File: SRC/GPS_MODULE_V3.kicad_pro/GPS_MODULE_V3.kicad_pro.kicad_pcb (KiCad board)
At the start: 4 copper layers, 50.1 x 41 mm, 141 parts, among them J1 Input, J3 nano_sim, J4 Micro_SD_Card, J5 Conn_02x06_Counter_Clockwise, Q1 SSM3J328R-HXY, Q2 BSN20, Q3 BSN20, Q4 2N7002, Q5 2N7002, Q6 2N7002, Q7 2N7002, U1 SY8089AAAC, U2 STM32F103C8Tx, U3 A9G_MODULE, U4 MAX485E, U5 XC6206PxxxMR, U7 ATA6561-GAQW-N, U8 W25Q32JVSS, Y1 8MHz, Y2 32.678KHz

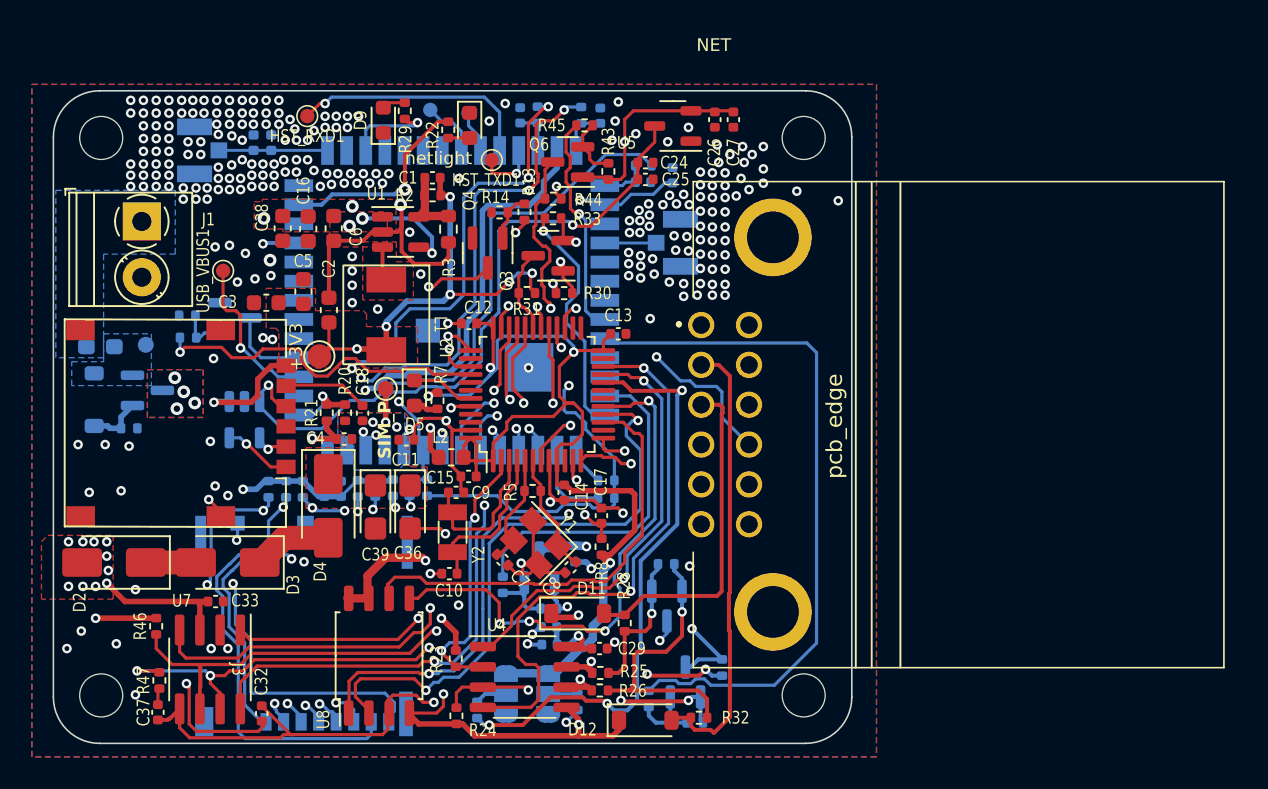
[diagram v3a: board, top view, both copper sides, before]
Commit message: completed GPS ecoboda files
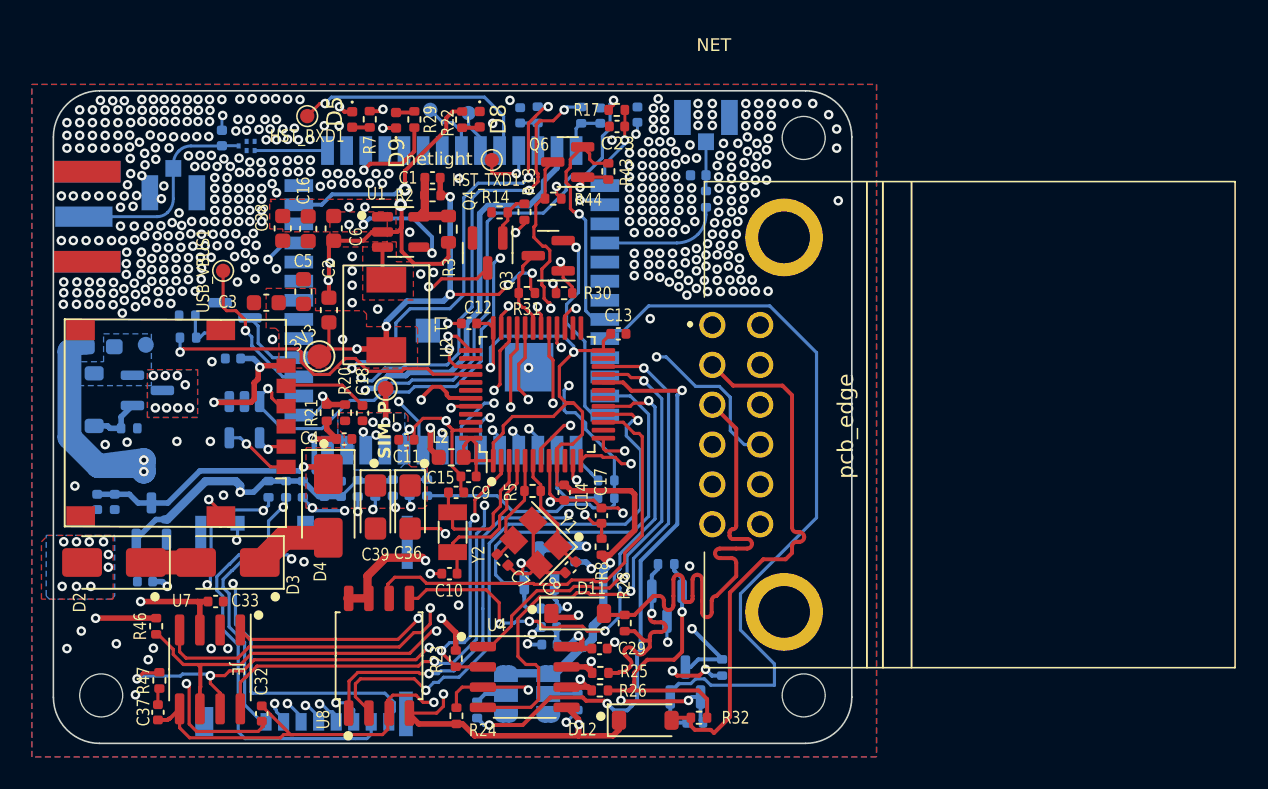
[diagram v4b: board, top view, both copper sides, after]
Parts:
- removed H2: MountingHole, MountingHole:MountingHole_2.7mm
- removed J1: Input, TerminalBlock_Phoenix:TerminalBlock_Phoenix_PT-1,5-2-3.5-H_1x02_P3.50mm_Horizontal
- removed R33, R36, R45, R50: 1K, Resistor_SMD:R_0402_1005Metric
- added AE3: Antenna_Shield, greencharge-footprints:UFL_COAX_CONN23370191, B.Cu at (230.9, 72.4)
- added C19: 0.1u, Capacitor_SMD:C_0402_1005Metric, B.Cu at (234.6, 82.8)
- added FL1: SAFEB1G57KE0F00R15, Filter:Filter_1411-5_1.4x1.1mm, B.Cu at (235.5, 69.5)
- added R51: 0R, Resistor_SMD:R_0402_1005Metric, B.Cu at (264.3, 72.8)
- AE1: footprint greencharge-footprints:UFL_COAX_CONN23370191 -> Connector_Coaxial:SMA_Samtec_SMA-J-P-X-ST-EM1_EdgeMount
- C23, R17: moved to F.Cu
- C24, C25, C26, C27, U5: moved to B.Cu
- D2, D3, D4: value SS310 -> RS1K-E3/5AT
- D5, D8, D9: footprint LED_SMD:LED_0603_1608Metric -> LED_SMD:LED_0402_1005Metric
- moved C27 46.9 mm to (229.1, 96.8), turned to 0 degrees
- moved C26 45.3 mm to (229.1, 95.6), turned to 0 degrees
- moved U5 41.1 mm to (229.5, 93.0), turned to 90 degrees
- moved C24 40.5 mm to (226.1, 91.8), turned to -90 degrees
- moved C25 39.0 mm to (227.2, 91.8), turned to -90 degrees
- moved G*** 35.0 mm to (261.3, 81.5)
- moved D6 28.0 mm to (263.8, 71.3), turned to 0 degrees
- moved R7 18.2 mm to (243.2, 67.8)
- moved D5 17.6 mm to (242.1, 67.8)
- moved G*** 10.6 mm to (270.2, 87.3)
- moved AE2 8.03 mm to (264.3, 67.7), turned to 180 degrees
- moved AE1 7.93 mm to (225.5, 73.9), turned to 90 degrees
- moved C20 4.39 mm to (260.0, 67.5)
- moved R17 3.87 mm to (258.7, 67.2), turned to 180 degrees
- moved C23 3.85 mm to (258.7, 68.2), turned to 180 degrees
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- renumbered J3 to JE
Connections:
- C16 pad 1: +5V -> /5V_FILTERED_
- C38 pad 1: +5V -> /5V_FILTERED_
- C6 pad 1: +5V -> /5V_FILTERED_
- D2 pad 2: +5V -> /5V_FILTERED_
- D6 pad 2: Net-(AE1-A) -> Net-(AE2-A)
- L3 pad 1: GND -> Net-(AE1-A)
- L3 pad 2: Net-(AE1-A) -> 4.2V_SIMPWR
- Q1 pad 3: +5V -> /5V_FILTERED_
- Q4 pad 2: Net-(Q4-S) -> /A9G_GSM_GPRS_MODULE/MOSFET_LOGIC_LEVEL_TRANSLATOR9/LOW_SIDE_LOGIC_SIGNAL
- Q5 pad 2: Net-(Q5-S) -> /A9G_GSM_GPRS_MODULE/MOSFET_LOGIC_LEVEL_TRANSLATOR6/LOW_SIDE_LOGIC_SIGNAL
- Q6 pad 2: Net-(Q6-S) -> /A9G_GSM_GPRS_MODULE/MOSFET_LOGIC_LEVEL_TRANSLATOR7/LOW_SIDE_LOGIC_SIGNAL
- Q7 pad 2: Net-(Q7-S) -> /A9G_GSM_GPRS_MODULE/MOSFET_LOGIC_LEVEL_TRANSLATOR8/LOW_SIDE_LOGIC_SIGNAL
- R30 pad 2: Net-(Q4-S) -> /A9G_GSM_GPRS_MODULE/MOSFET_LOGIC_LEVEL_TRANSLATOR9/LOW_SIDE_LOGIC_SIGNAL
- R34 pad 2: Net-(Q5-S) -> /A9G_GSM_GPRS_MODULE/MOSFET_LOGIC_LEVEL_TRANSLATOR6/LOW_SIDE_LOGIC_SIGNAL
- R43 pad 2: Net-(Q6-S) -> /A9G_GSM_GPRS_MODULE/MOSFET_LOGIC_LEVEL_TRANSLATOR7/LOW_SIDE_LOGIC_SIGNAL
- R48 pad 2: Net-(Q7-S) -> /A9G_GSM_GPRS_MODULE/MOSFET_LOGIC_LEVEL_TRANSLATOR8/LOW_SIDE_LOGIC_SIGNAL
- TH1 pad 1: Net-(J1-Pin_1) -> +5V
- U1 pad 1: +5V -> /5V_FILTERED_
- U1 pad 4: +5V -> /5V_FILTERED_
- U2 pad 32: /CAN_TRANSCEIVER_ATA6561/CAN_TX -> /CAN_TRANSCEIVER_ATA6561/CAN_RX
- U2 pad 33: /CAN_TRANSCEIVER_ATA6561/CAN_RX -> /CAN_TRANSCEIVER_ATA6561/CAN_TX
- U3 pad 28: Net-(AE1-A) -> Net-(U3-GPS_RF)
- U3 pad 45: Net-(AE2-A) -> Net-(U3-GSM_RF)
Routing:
- net Net-(D5-K): track 4.00 -> 39.8 mm, vias 0 -> 2
- net 4.2V_SIMPWR: track 33.9 -> 59.1 mm, vias 6 -> 8
- net /STM32F103C8T6_MCU/3v3_stm: track 66.9 -> 86.4 mm
- net /RS485_MAX485/B: track 21.0 -> 34.1 mm
- net Net-(U3-GSM_RF): track 0.00 -> 7.82 mm
- net /5V_FILTERED_: track 0.00 -> 7.37 mm, vias 0 -> 22
- net GND: track 102.1 -> 109.2 mm, vias 253 -> 462
- net Net-(Q4-S): track 6.74 -> 0.00 mm, vias 2 -> 0
- net B_to_CANH: track 36.9 -> 43.5 mm
- net Net-(AE1-A): track 6.82 -> 13.3 mm
- net /RS485_MAX485/A: track 28.4 -> 34.2 mm
- net /A9G_GSM_GPRS_MODULE/MOSFET_LOGIC_LEVEL_TRANSLATOR8/LOW_SIDE_LOGIC_SIGNAL: track 21.2 -> 26.3 mm
- net Net-(Q5-S): track 4.78 -> 0.00 mm
- net /A9G_GSM_GPRS_MODULE/MOSFET_LOGIC_LEVEL_TRANSLATOR6/LOW_SIDE_LOGIC_SIGNAL: track 44.1 -> 48.8 mm
- net Net-(U3-GPS_RF): track 0.00 -> 4.58 mm
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- added copper zone on B.Cu, net /5V_FILTERED_
- added copper zone on F.Cu, net /5V_FILTERED_
- added copper zone on In2.Cu, net /5V_FILTERED_
- removed copper zone on B.Cu, net +5V
- removed copper zone on F.Cu, net +5V
- removed copper zone on In2.Cu, net +5V
- removed copper zone on B.Cu, net Net-(J1-Pin_1)
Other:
- board text added: "3V3"
- board text removed: "+3V3"
